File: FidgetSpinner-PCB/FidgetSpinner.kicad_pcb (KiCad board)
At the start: 2 copper layers, 80.5 x 88.6 mm, 37 parts, among them J1 EdgeConnector, J2 GP2S27, SW1 SW_POWER, SW2 button, U1 STM32L010K8T6

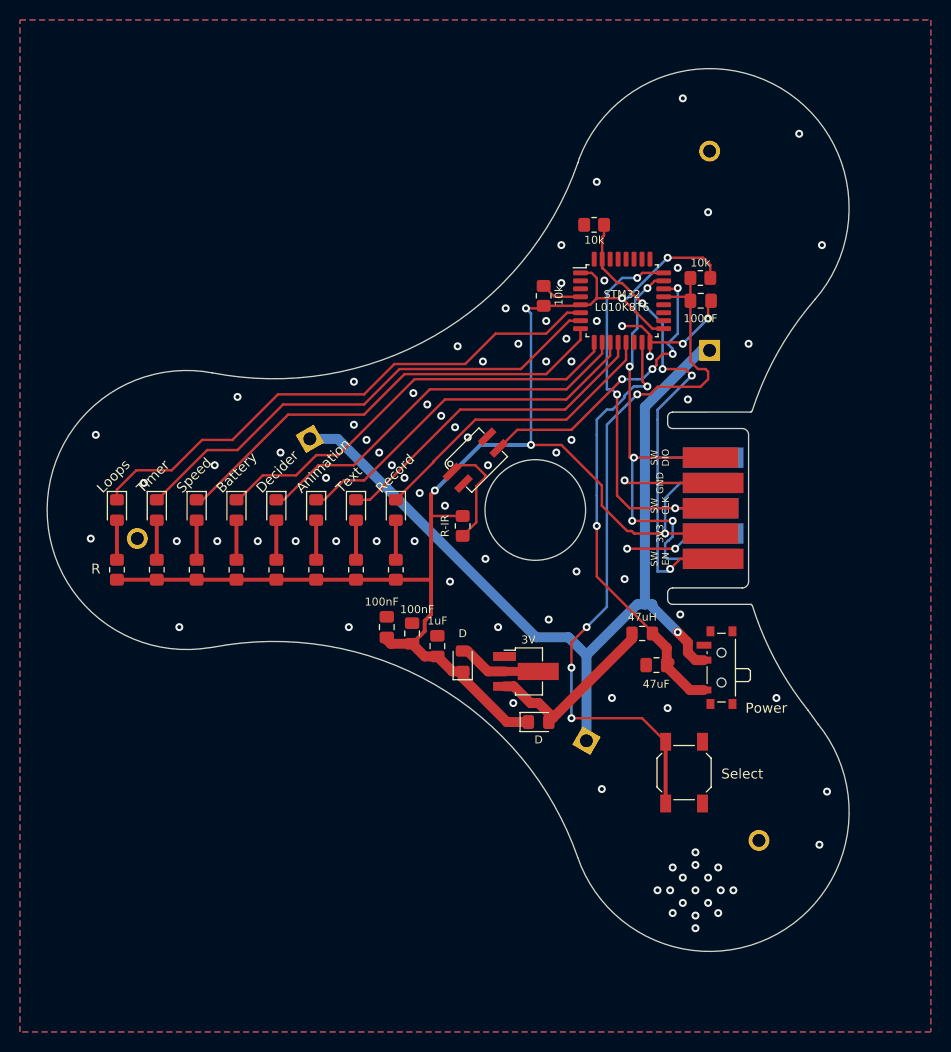
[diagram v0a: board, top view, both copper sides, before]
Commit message: important updates
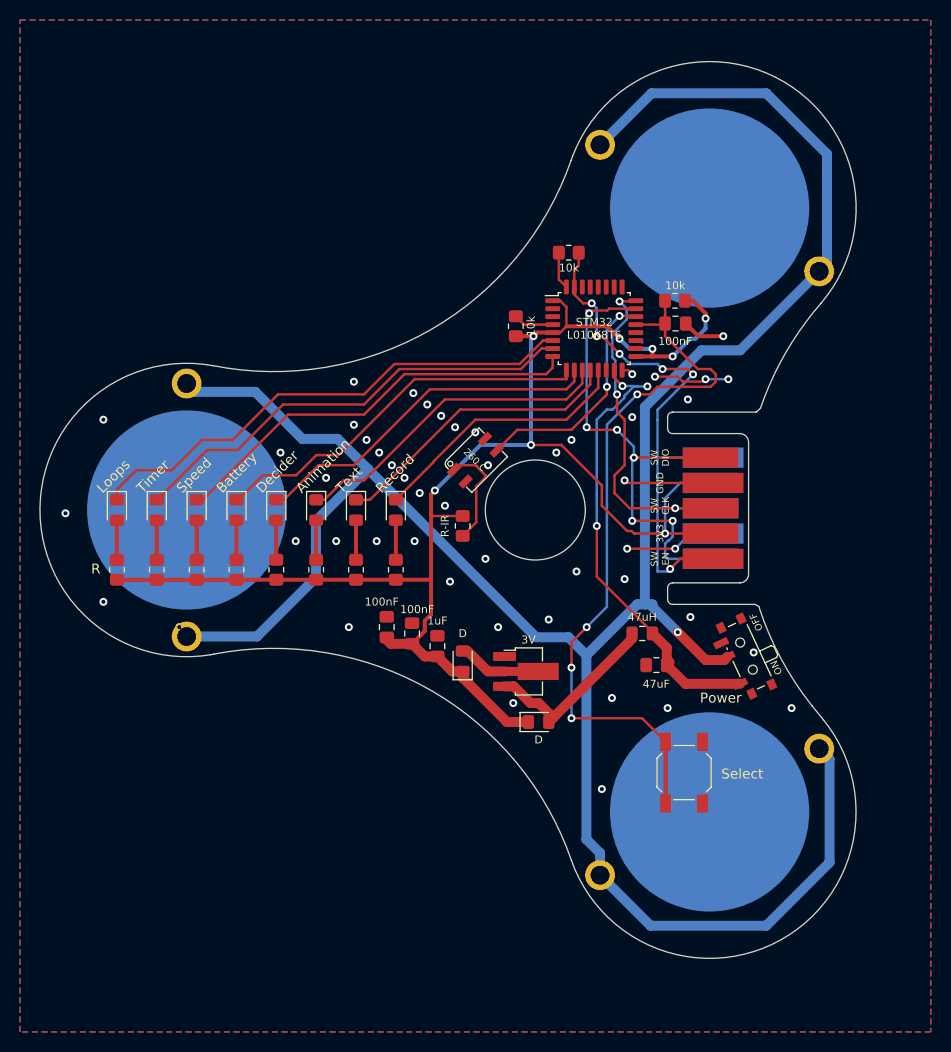
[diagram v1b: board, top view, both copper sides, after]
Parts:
- BT1, BT2, BT3: value CR2032 -> CR2450; footprint WYW_Package:CR2450_Centered -> Battery:BatteryHolder_Keystone_3009_1x2450
- moved R12 4.13 mm to (98.0, 81.5)
- moved U1 3.95 mm to (105.9, 81.8)
- moved R11 3.78 mm to (103.4, 74.2)
- moved C8 3.42 mm to (114.1, 81.3)
- moved R9 3.42 mm to (114.0, 79.0)
- moved SW1 2.74 mm to (120.9, 114.8), turned to 115 degrees
- turned BT1 to 270 degrees
- turned BT2 to 30 degrees
- turned BT3 to 150 degrees
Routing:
- net Net-(BT1-Pad1): track 91.0 -> 243.6 mm, vias 1 -> 2
- net ~INT_C: track 30.4 -> 23.5 mm, vias 4 -> 2
- net SWCLK: track 41.1 -> 36.6 mm
- net L1: track 50.0 -> 46.0 mm
- net L0: track 54.9 -> 51.0 mm
- net L2: track 46.3 -> 42.4 mm
- net L7: track 30.7 -> 26.8 mm
- net L6: track 33.7 -> 29.7 mm
- net L5: track 36.8 -> 32.9 mm
- net L4: track 39.9 -> 36.0 mm
- net L3: track 43.0 -> 39.0 mm
- net SWDIO: track 47.1 -> 50.8 mm, vias 5 -> 6
- net VCC: track 158.0 -> 155.3 mm, vias 6 -> 8
- net GND: track 32.4 -> 35.2 mm, vias 90 -> 49
- net VBAT: track 44.1 -> 45.9 mm, vias 2 -> 3
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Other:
- board size 80.5 x 88.6 mm -> 81.9 x 90 mm
- board text added: "260.C"
- board text added: "OFF"
- board text added: "ON"
- board text added: "PhOVS FidgetSpinner v0.4.1 - (C) WYW 2021-11-08"
- board text removed: "PhOVS FidgetSpinner v0.2.0 - (C) WYW 2021-11-08"
